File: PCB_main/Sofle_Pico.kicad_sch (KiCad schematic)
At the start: 68 parts, among them J1 Conn_02x08_Top_Bottom, J2 Conn_02x08_Top_Bottom, J3 Conn_01x06, SW1 SW_PUSH, SW10 SW_PUSH, SW11 SW_PUSH, SW12 SW_PUSH, SW13 SW_PUSH, SW14 SW_PUSH, SW15 SW_PUSH, SW16 SW_PUSH, SW17 SW_PUSH, SW18 SW_PUSH, SW2 SW_PUSH, SW20 SW_PUSH, SW21 SW_PUSH, SW22 SW_PUSH, SW23 SW_PUSH, SW24 SW_PUSH, SW27 SW_PUSH, SW28 SW_PUSH, SW29 SW_PUSH, SW3 SW_PUSH, SW30 SW_PUSH, SW37 SW_PUSH, SW38 SW_PUSH, SW39 SW_PUSH, SW4 SW_PUSH, SW40 SW_PUSH, SW41 SW_PUSH, SW5 SW_PUSH, SW6 SW_PUSH, SW7 SW_PUSH, SW8 SW_PUSH, SW9 SW_PUSH, U2 Pico

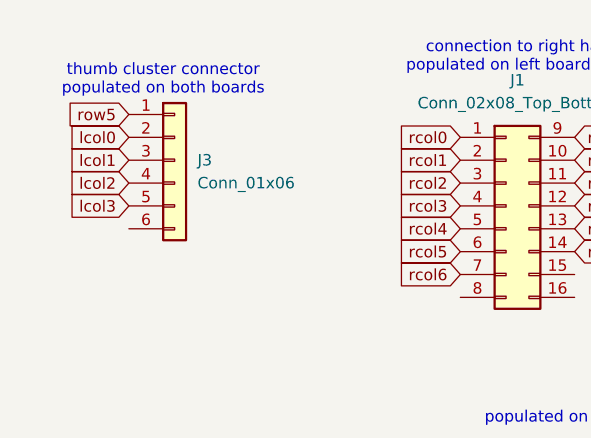
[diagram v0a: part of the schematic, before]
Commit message: improve positioning
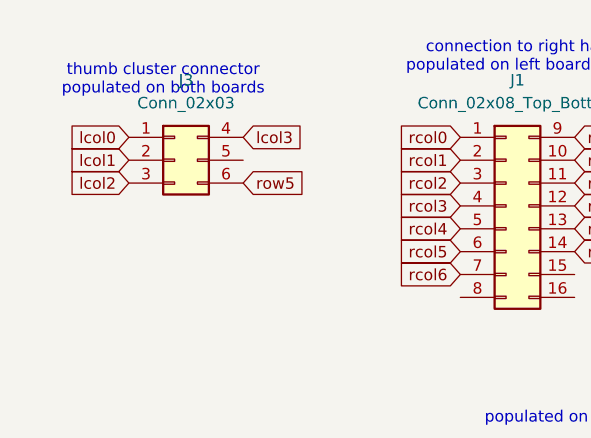
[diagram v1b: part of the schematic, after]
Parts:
- J3: value Conn_01x06 -> Conn_02x03; footprint Connector_PinHeader_1.27mm:PinHeader_1x06_P1.27mm_Horizontal -> Connector_PinHeader_2.54mm:PinHeader_2x03_P2.54mm_Vertical; symbol Connector_Generic:Conn_01x06 -> Connector_Generic:Conn_02x03_Top_Bottom
- U2: footprint Module:RaspberryPi_Pico_SMD_HandSolder -> Module:RaspberryPi_Pico_SMD
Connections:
- net lcol0: now also J3.1 (Pin_1); no longer J3.2 (Pin_2)
- net lcol1: now also J3.2 (Pin_2); no longer J3.3 (Pin_3)
- net lcol2: now also J3.3 (Pin_3); no longer J3.4 (Pin_4)
- net lcol3: now also J3.4 (Pin_4); no longer J3.5 (Pin_5)
- net row5: now also J3.6 (Pin_6); no longer J3.1 (Pin_1)
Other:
- moved on the sheet: J3
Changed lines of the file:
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@@
 	(global_label "row5"
 		(shape input)
-		(at 31.75 31.75 180)
+		(at 44.45 39.37 0)
 		(effects
 			(font
 				(size 1.27 1.27)
 			)
-			(justify right)
+			(justify left)
 		)
 		(property "Intersheetrefs" "${INTERSHEET_REFS}"
-			(at 31.75 31.75 0)
+			(at 44.45 39.37 0)
 			(effects
 				(font
@@
 	(global_label "lcol3"
 		(shape input)
-		(at 31.75 41.91 180)
+		(at 44.45 34.29 0)
 		(effects
 			(font
 				(size 1.27 1.27)
 			)
-			(justify right)
+			(justify left)
 		)
 		(property "Intersheetrefs" "${INTERSHEET_REFS}"
-			(at 31.75 41.91 90)
+			(at 44.45 34.29 90)
 			(effects
 				(font
@@
 			)
 		)
-		(property "Footprint" "Module:RaspberryPi_Pico_SMD_HandSolder"
+		(property "Footprint" "Module:RaspberryPi_Pico_SMD"
 			(at 217.17 105.41 90)
 			(effects
@@
 	)
 	(symbol
-		(lib_id "Connector_Generic:Conn_01x06")
+		(lib_id "Connector_Generic:Conn_02x03_Top_Bottom")
 		(at 36.83 36.83 0)
 		(unit 1)
@@
 		(fields_autoplaced yes)
 		(property "Reference" "J3"
-			(at 39.37 36.8299 0)
+			(at 38.1 27.94 0)
 			(effects
 				(font
 					(size 1.27 1.27)
 				)
-				(justify left)
 			)
 		)
-		(property "Value" "Conn_01x06"
-			(at 39.37 39.3699 0)
+		(property "Value" "Conn_02x03"
+			(at 38.1 30.48 0)
 			(effects
 				(font
 					(size 1.27 1.27)
 				)
-				(justify left)
 			)
 		)
-		(property "Footprint" "Connector_PinHeader_1.27mm:PinHeader_1x06_P1.27mm_Horizontal"
+		(property "Footprint" "Connector_PinHeader_2.54mm:PinHeader_2x03_P2.54mm_Vertical"
 			(at 36.83 36.83 0)
 			(effects
@@
 			)
 		)
-		(property "Description" "Generic connector, single row, 01x06, script generated (kicad-library-utils/schlib/autogen/connector/)"
+		(property "Description" "Generic connector, double row, 02x03, top/bottom pin numbering scheme (row 1: 1...pins_per_row, row2: pins_per_row+1 ... num_pins), script generated (kicad-library-utils/schlib/autogen/connector/)"
 			(at 36.83 36.83 0)
 			(effects

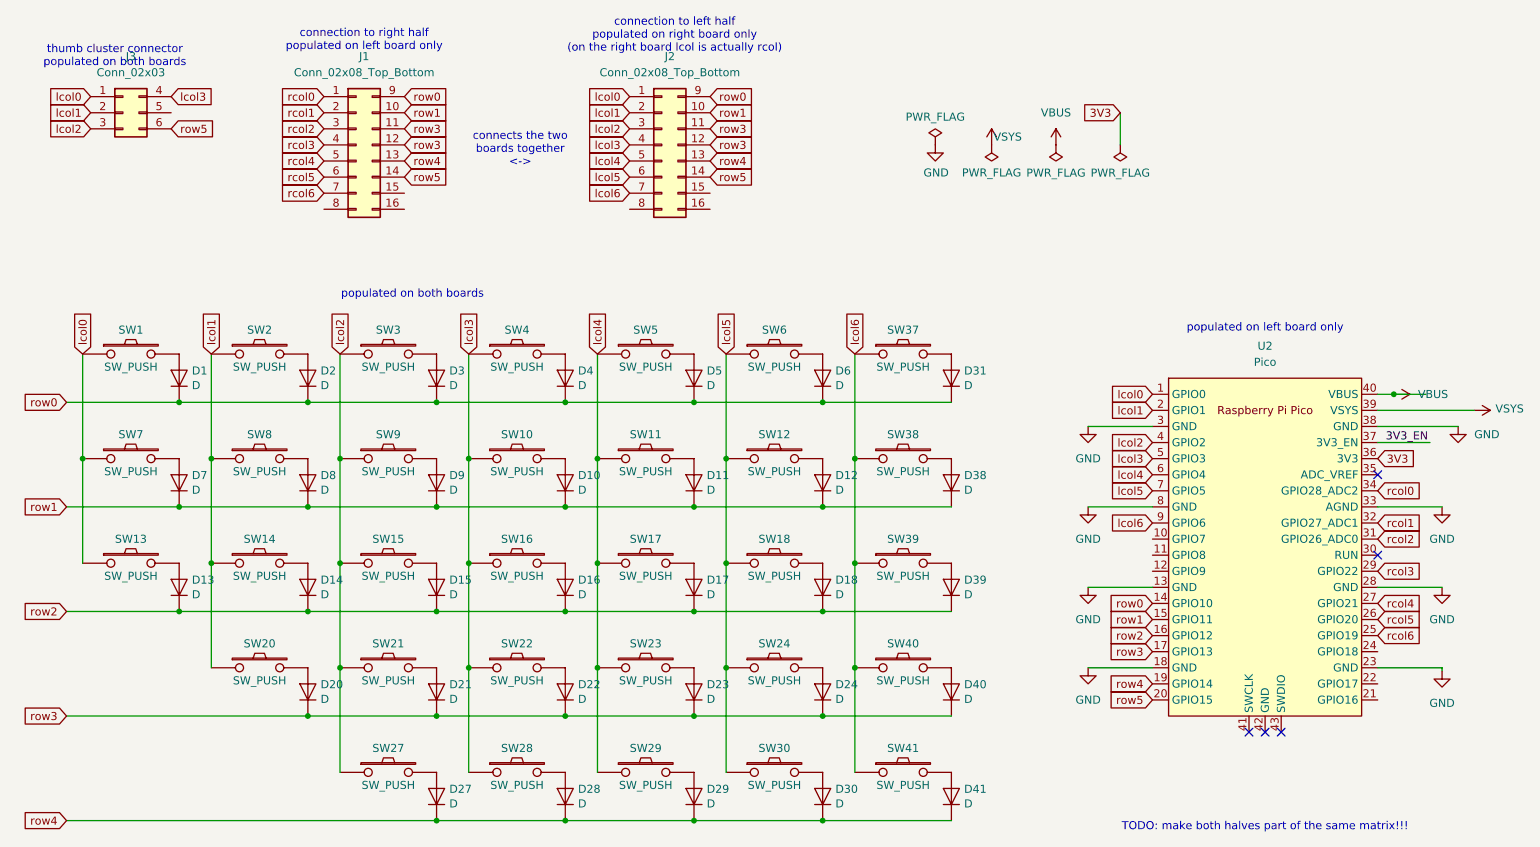
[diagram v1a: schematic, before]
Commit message: more pcb progress
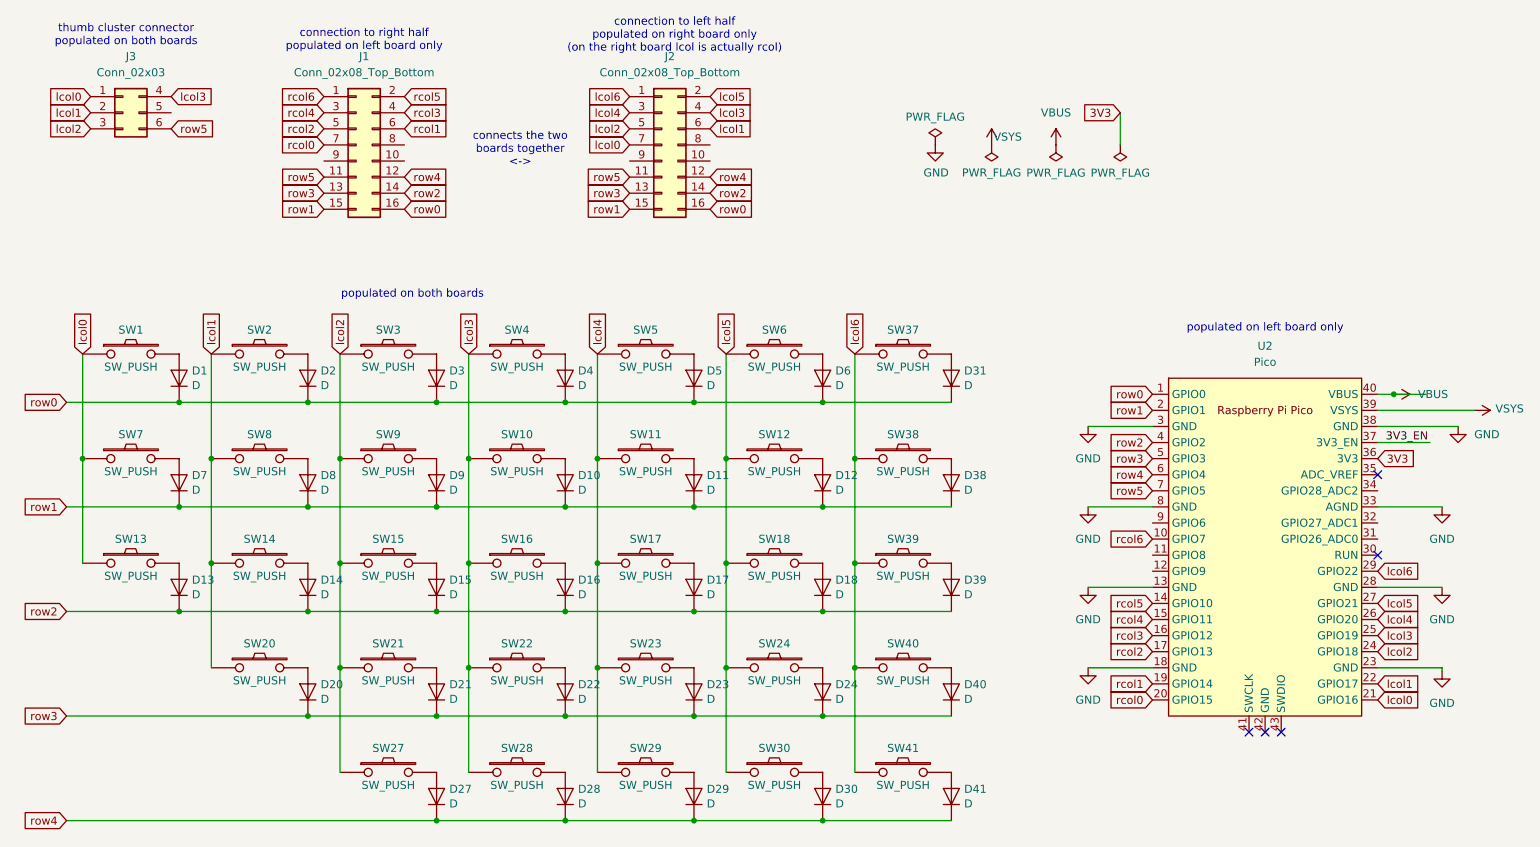
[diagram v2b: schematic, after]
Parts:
- J1, J2: footprint Connector_PinHeader_1.27mm:PinHeader_2x08_P1.27mm_Horizontal -> Connector_PinHeader_2.00mm:PinHeader_2x08_P2.00mm_Vertical; symbol Connector_Generic:Conn_02x08_Top_Bottom -> Connector_Generic:Conn_02x08_Odd_Even
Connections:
- net lcol0: now also J2.7 (Pin_7), U2.21 (GPIO16); no longer J2.1 (Pin_1), U2.1 (GPIO0)
- net lcol1: now also J2.6 (Pin_6), U2.22 (GPIO17); no longer J2.2 (Pin_2), U2.2 (GPIO1)
- net lcol2: now also J2.5 (Pin_5), U2.24 (GPIO18); no longer J2.3 (Pin_3), U2.4 (GPIO2)
- net lcol3: now also U2.25 (GPIO19); no longer U2.5 (GPIO3)
- net lcol4: now also J2.3 (Pin_3), U2.26 (GPIO20); no longer J2.5 (Pin_5), U2.6 (GPIO4)
- net lcol5: now also J2.2 (Pin_2), U2.27 (GPIO21); no longer J2.6 (Pin_6), U2.7 (GPIO5)
- net lcol6: now also J2.1 (Pin_1), U2.29 (GPIO22); no longer J2.7 (Pin_7), U2.9 (GPIO6)
- net rcol0: now also J1.7 (Pin_7), U2.20 (GPIO15); no longer J1.1 (Pin_1), U2.34 (GPIO28_ADC2)
- net rcol1: now also J1.6 (Pin_6), U2.19 (GPIO14); no longer J1.2 (Pin_2), U2.32 (GPIO27_ADC1)
- net rcol2: now also J1.5 (Pin_5), U2.17 (GPIO13); no longer J1.3 (Pin_3), U2.31 (GPIO26_ADC0)
- net rcol3: now also U2.16 (GPIO12); no longer U2.29 (GPIO22)
- net rcol4: now also J1.3 (Pin_3), U2.15 (GPIO11); no longer J1.5 (Pin_5), U2.27 (GPIO21)
- net rcol5: now also J1.2 (Pin_2), U2.14 (GPIO10); no longer J1.6 (Pin_6), U2.26 (GPIO20)
- net rcol6: now also J1.1 (Pin_1), U2.10 (GPIO7); no longer J1.7 (Pin_7), U2.25 (GPIO19)
- net row0: now also J1.16 (Pin_16), J2.16 (Pin_16), U2.1 (GPIO0); no longer J1.9 (Pin_9), J2.9 (Pin_9), U2.14 (GPIO10)
- net row1: now also J1.15 (Pin_15), J2.15 (Pin_15), U2.2 (GPIO1); no longer J1.10 (Pin_10), J2.10 (Pin_10), U2.15 (GPIO11)
- net row2: now also J1.14 (Pin_14), J2.14 (Pin_14), U2.4 (GPIO2); no longer U2.16 (GPIO12)
- net row3: now also J1.13 (Pin_13), J2.13 (Pin_13), U2.5 (GPIO3); no longer J1.11 (Pin_11), J1.12 (Pin_12), J2.11 (Pin_11), J2.12 (Pin_12), U2.17 (GPIO13)
- net row4: now also J1.12 (Pin_12), J2.12 (Pin_12), U2.6 (GPIO4); no longer J1.13 (Pin_13), J2.13 (Pin_13), U2.19 (GPIO14)
- net row5: now also J1.11 (Pin_11), J2.11 (Pin_11), U2.7 (GPIO5); no longer J1.14 (Pin_14), J2.14 (Pin_14), U2.20 (GPIO15)
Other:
- note removed: "TODO: make both halves part of the same matrix!!!"

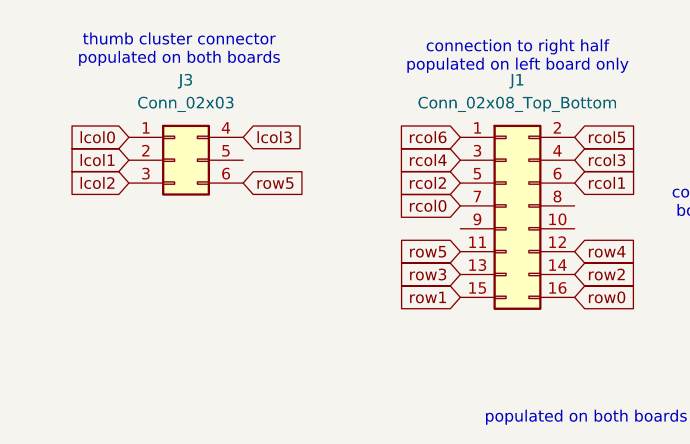
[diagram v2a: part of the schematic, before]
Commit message: more
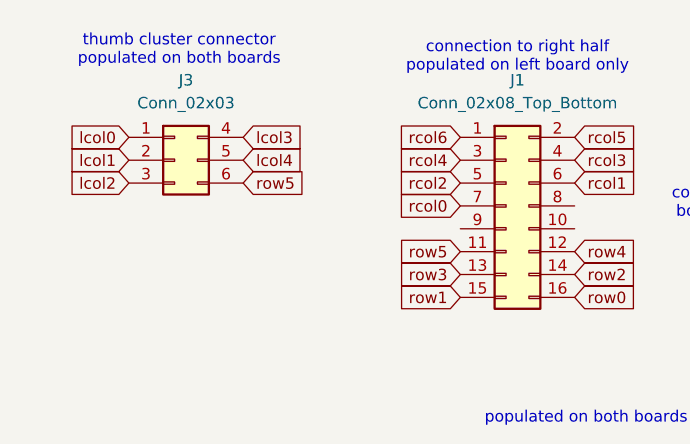
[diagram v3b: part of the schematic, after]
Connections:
- net lcol4: now also J3.5 (Pin_5)
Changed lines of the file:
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@@
+		)
+	)
+	(global_label "lcol4"
+		(shape input)
+		(at 44.45 36.83 0)
+		(effects
+			(font
+				(size 1.27 1.27)
+			)
+			(justify left)
+		)
+		(property "Intersheetrefs" "${INTERSHEET_REFS}"
+			(at 44.45 36.83 0)
+			(effects
+				(font
+					(size 1.27 1.27)
+				)
+				(hide yes)
+			)
 		)
 	)
